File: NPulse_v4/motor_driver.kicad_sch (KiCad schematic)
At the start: 96 parts, among them IC2 DRV8220DSGR, IC3 DRV8220DSGR, IC4 DRV8220DSGR, IC5 DRV8220DSGR, IC6 DRV8220DSGR, IC7 DRV8220DSGR, IC8 DRV8220DSGR, IC9 DRV8220DSGR, J6 Conn_02x05_Odd_Even, J7 Conn_02x05_Odd_Even, J8 Conn_02x05_Odd_Even, J9 Conn_02x05_Odd_Even, U2 SN74LVC002, U3 SN74LVC002, U4 SN74LVC002, U5 SN74LVC002, U6 SN74LVC002, U7 SN74LVC002, U8 SN74LVC002, U9 SN74LVC002

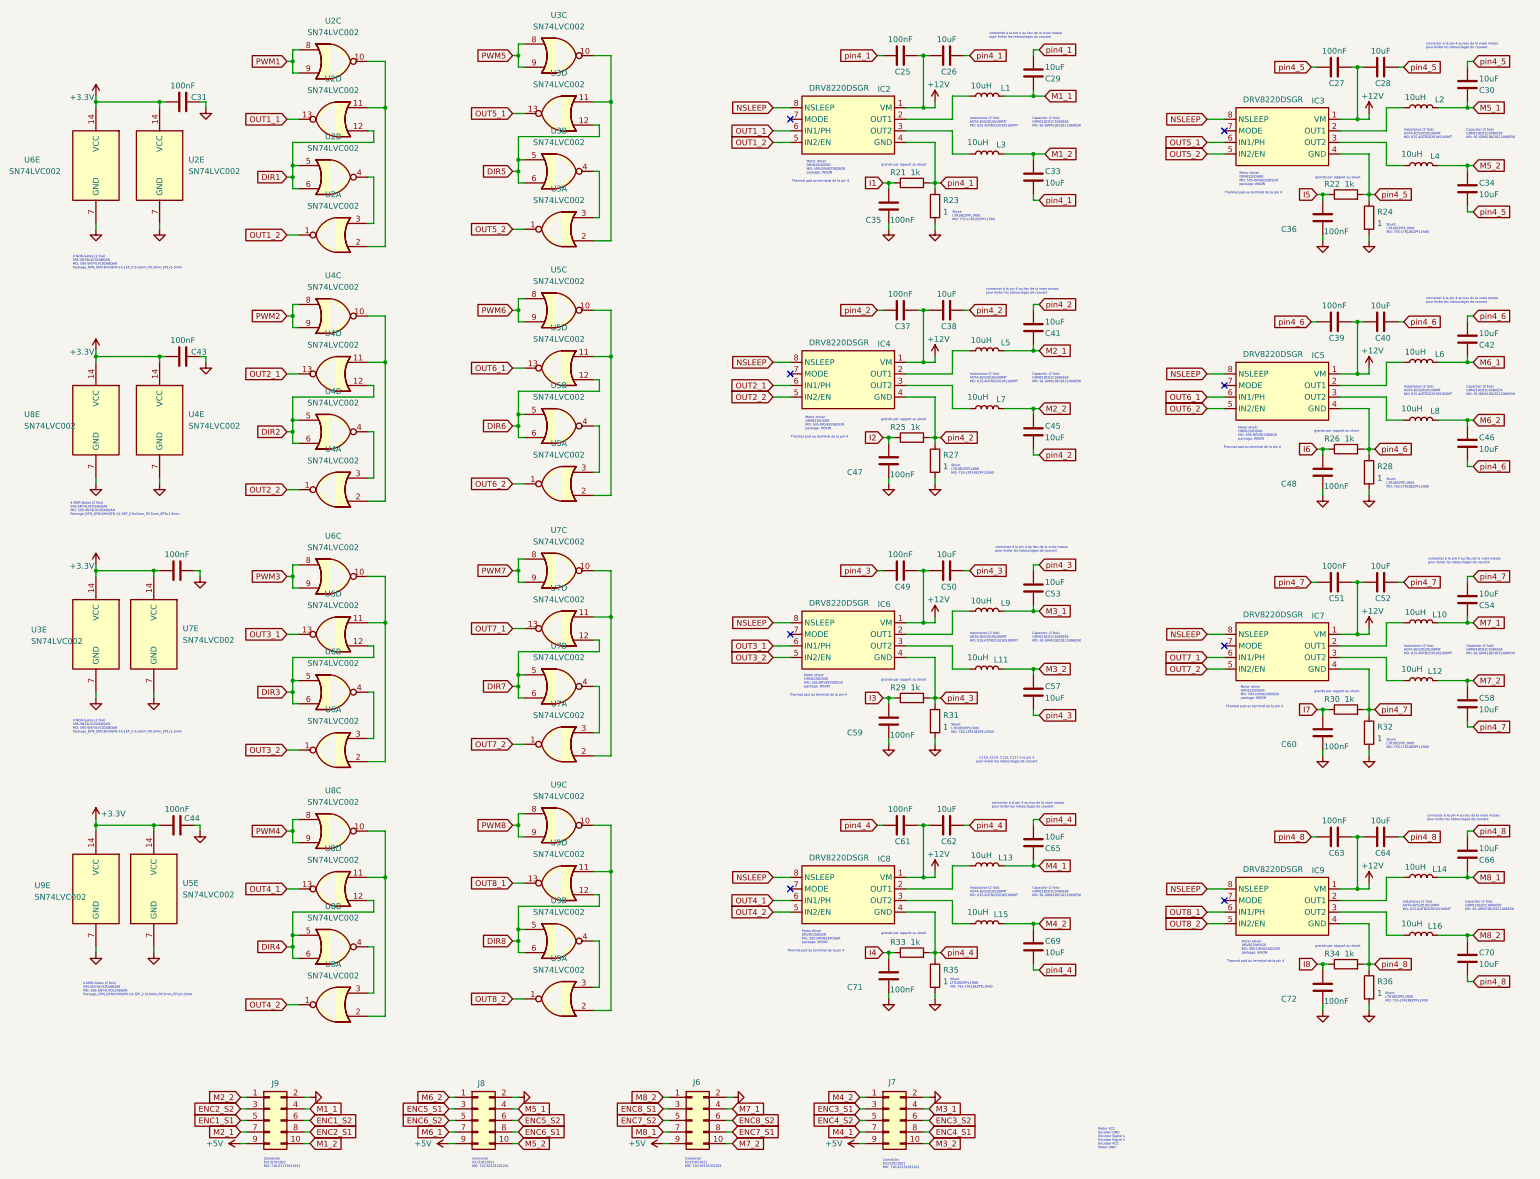
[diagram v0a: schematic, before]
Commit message: some modifications on the routing
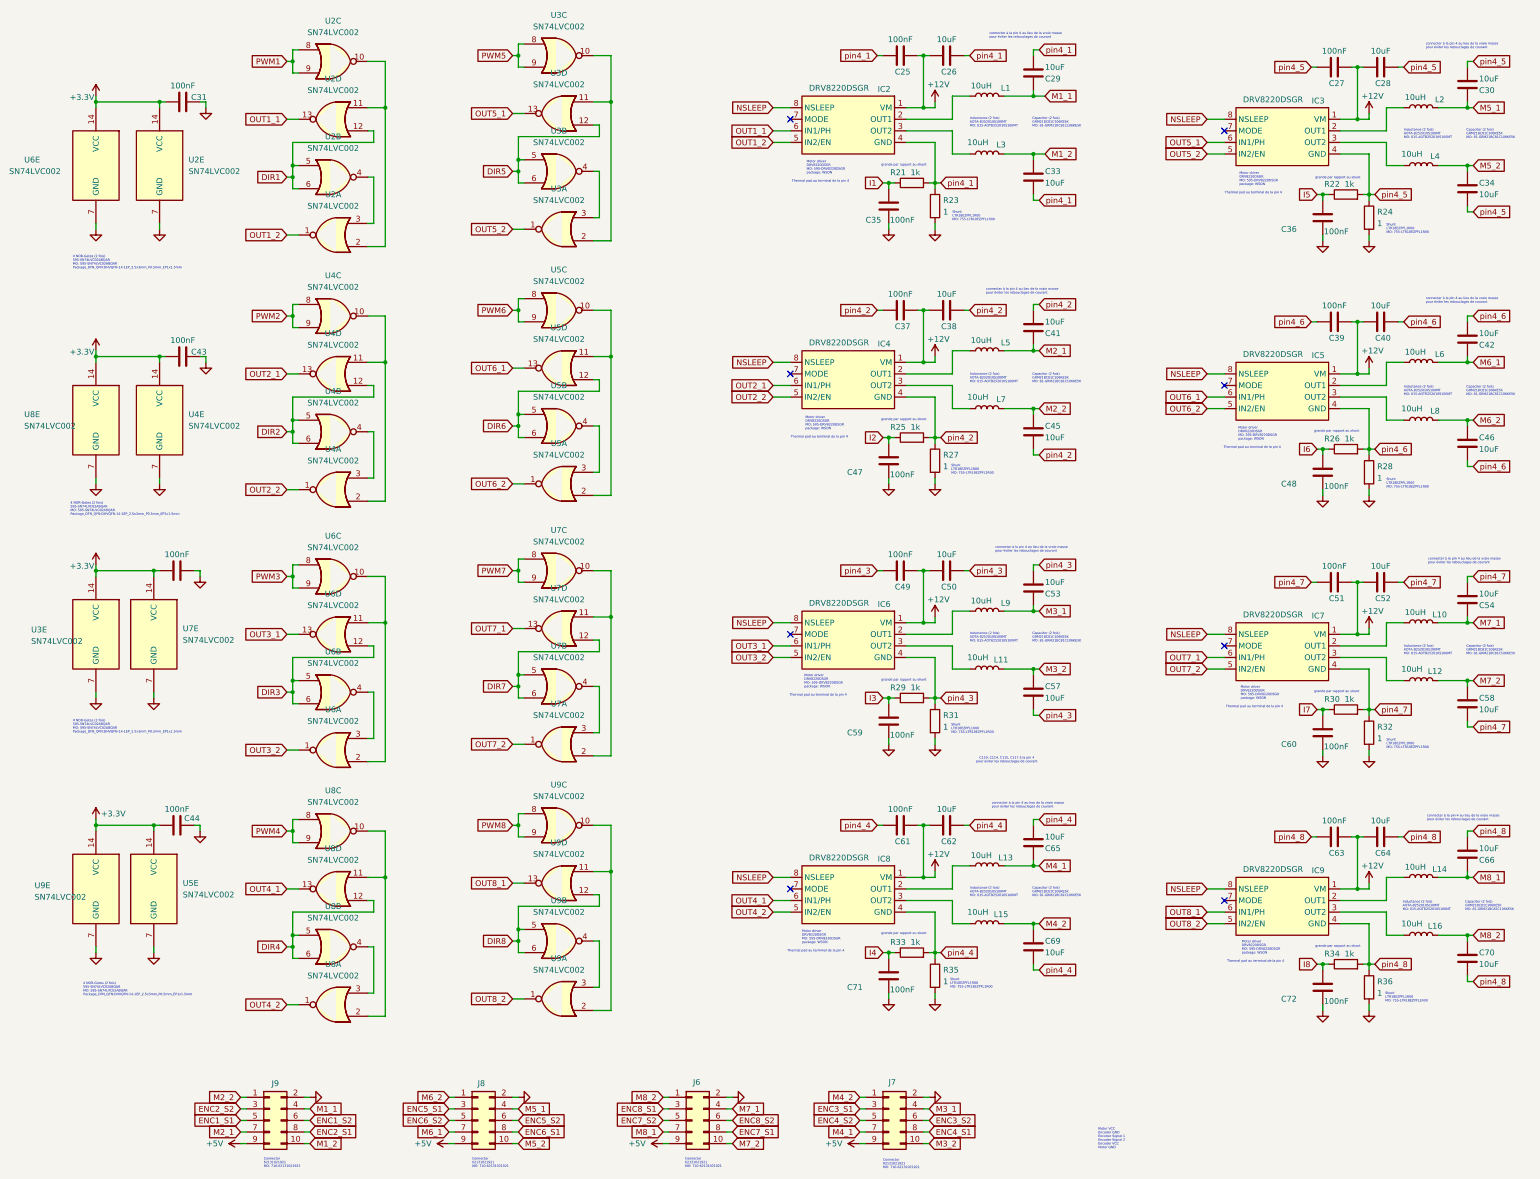
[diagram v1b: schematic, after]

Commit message: Few corrections: tracks, via, thermal pad
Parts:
- IC4: footprint DRV8220DSGR:WSON8_DSG_TEX -> SON50P200X200X80-9N
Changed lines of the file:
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@@
 	(wire
 		(pts
-			(xy 222.25 102.87) (xy 228.6 102.87)
-		)
-		(stroke
-			(width 0)
-			(type default)
-		)
-	)
-	(wire
-		(pts
 			(xy 323.85 41.91) (xy 321.31 41.91)
 		)
@@
 	(wire
 		(pts
+			(xy 222.25 102.87) (xy 228.6 102.87)
+		)
+		(stroke
+			(width 0)
+			(type default)
+		)
+	)
+	(wire
+		(pts
 			(xy 154.94 214.63) (xy 137.16 214.63)
 		)
@@
 	)
 	(symbol
+		(lib_name "DRV8220DSGR_1")
 		(lib_id "new_components:DRV8220DSGR")
 		(at 224.79 95.25 0)
@@
 			)
 		)
-		(property "Footprint" "DRV8220DSGR:WSON8_DSG_TEX"
+		(property "Footprint" "SON50P200X200X80-9N"
 			(at 198.12 190.17 0)
 			(effects

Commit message: Correct LDO schematic and update connectors to through-hole footprints
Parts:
- IC4: footprint SON50P200X200X80-9N -> DRV8220DSGR:WSON8_DSG_TEX
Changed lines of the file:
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@@
 			)
 		)
-		(property "Footprint" "SON50P200X200X80-9N"
+		(property "Footprint" "DRV8220DSGR:WSON8_DSG_TEX"
 			(at 198.12 190.17 0)
 			(effects
